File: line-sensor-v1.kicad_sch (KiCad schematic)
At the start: 1 part

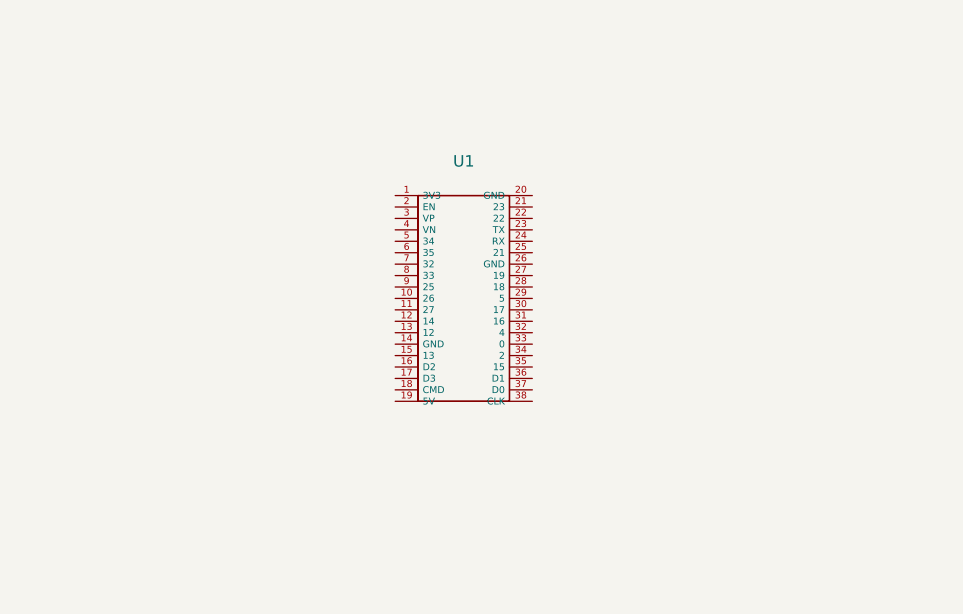
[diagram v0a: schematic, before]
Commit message: commit
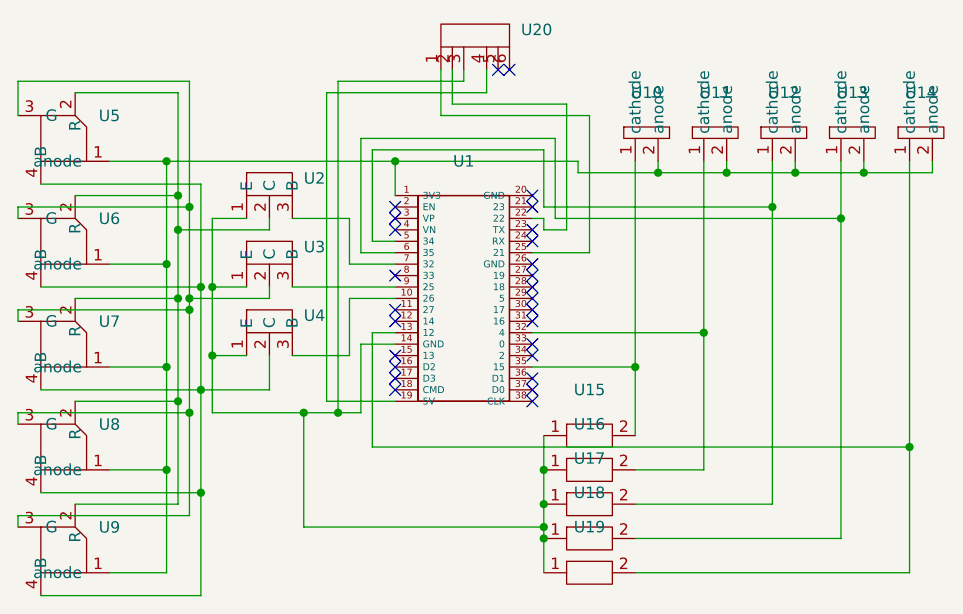
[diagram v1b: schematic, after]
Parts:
- added U10, U11, U12, U13, U14: ~, my-library:フォトトランジスタ, symbol my-library:フォトトランジスタ
- added U15, U16, U17, U18, U19: ~, my-library:resistance, symbol my-library:resistance
- added U2, U3, U4: ~, my-library:トランジスタ, symbol my-library:トランジスタ
- added U20: ~, my-library:6-pin, symbol my-library:6-pin
- added U5, U6, U7, U8, U9: ~, my-library:OSTBMAZ2C1D-LED, symbol my-library:OSTBMAZ2C1D-LED
- U1: footprint (none) -> my-library:ESP32-DevKitC-32E
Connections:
- net at U1.1 (3V3): now also U10.2 (anode), U11.2 (anode), U12.2 (anode), U13.2 (anode), U14.2 (anode), U5.1 (anode), U6.1 (anode), U7.1 (anode), U8.1 (anode), U9.1 (anode)
- net at U1.10 (26): now also U4.3 (B)
- net at U1.13 (12): now also U14.1 (cathode), U19.2
- net at U1.14 (GND): now also U15.1, U16.1, U17.1, U18.1, U19.1, U2.1 (E), U20.3, U3.1 (E), U4.1 (E)
- net at U1.19 (5V): now also U20.4
- net at U1.22: now also U20.2
- net at U1.25 (21): now also U20.1
- net at U1.32 (4): now also U11.1 (cathode), U16.2
- net at U1.35 (15): now also U10.1 (cathode), U15.2
- net at U1.5 (34): now also U12.1 (cathode), U17.2
- net at U1.6 (35): now also U13.1 (cathode), U18.2
- net at U1.7 (32): now also U2.3 (B)
- net at U1.9 (25): now also U3.3 (B)
- new net: U4.2 (C), U5.4 (B), U6.4 (B), U7.4 (B), U8.4 (B), U9.4 (B)
- new net: U2.2 (C), U5.2 (R), U6.2 (R), U7.2 (R), U8.2 (R), U9.2 (R)
- new net: U3.2 (C), U5.3 (G), U6.3 (G), U7.3 (G), U8.3 (G), U9.3 (G)
- no-connect marks 0 -> 27
